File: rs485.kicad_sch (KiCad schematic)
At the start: 4 parts, among them J1 Conn_01x04_Pin, J2 Conn_01x04_Socket, U2 SN74CB3Q3384APW

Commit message: sch of.
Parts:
- removed J2: Conn_01x04_Socket, symbol Connector:Conn_01x04_Socket
- added J2: Conn_01x04_Pin, symbol Connector:Conn_01x04_Pin
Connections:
- net GND: now also J2.1 (Pin_1); no longer J1.4 (Pin_4)
- net at U2.1 (~{1OE}): now also J1.3 (Pin_3)
- net at U2.13 (~{2OE}): now also J1.4 (Pin_4)
- net at U2.2 (1B1): now also J1.1 (Pin_1)
- net at U1.1 (R), U1.4 (D): now also U2.4 (1A2); no longer U2.3 (1A1)
- net at U1.2 (RE~), U1.3 (DE): now also U2.3 (1A1); no longer U2.4 (1A2)
- net at U2.5 (1B2): now also J1.2 (Pin_2)
- net at U1.6 (B): now also J2.3 (Pin_3); no longer J1.2 (Pin_2)
- net at U1.7 (A): now also J2.4 (Pin_4); no longer J1.1 (Pin_1)
- net +5V renamed VCC
- net VCC: now also J2.2 (Pin_2); no longer J1.3 (Pin_3)

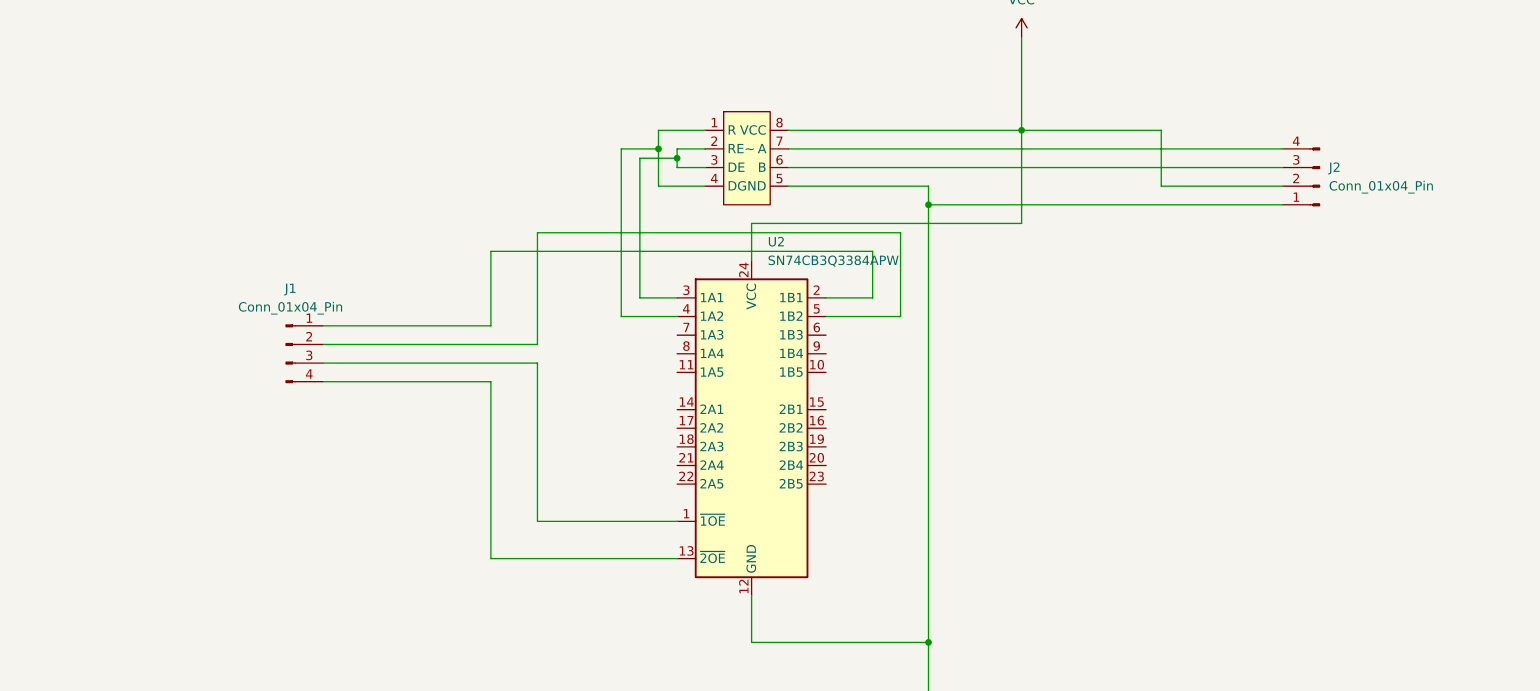
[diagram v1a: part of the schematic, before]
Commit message: sch ok.
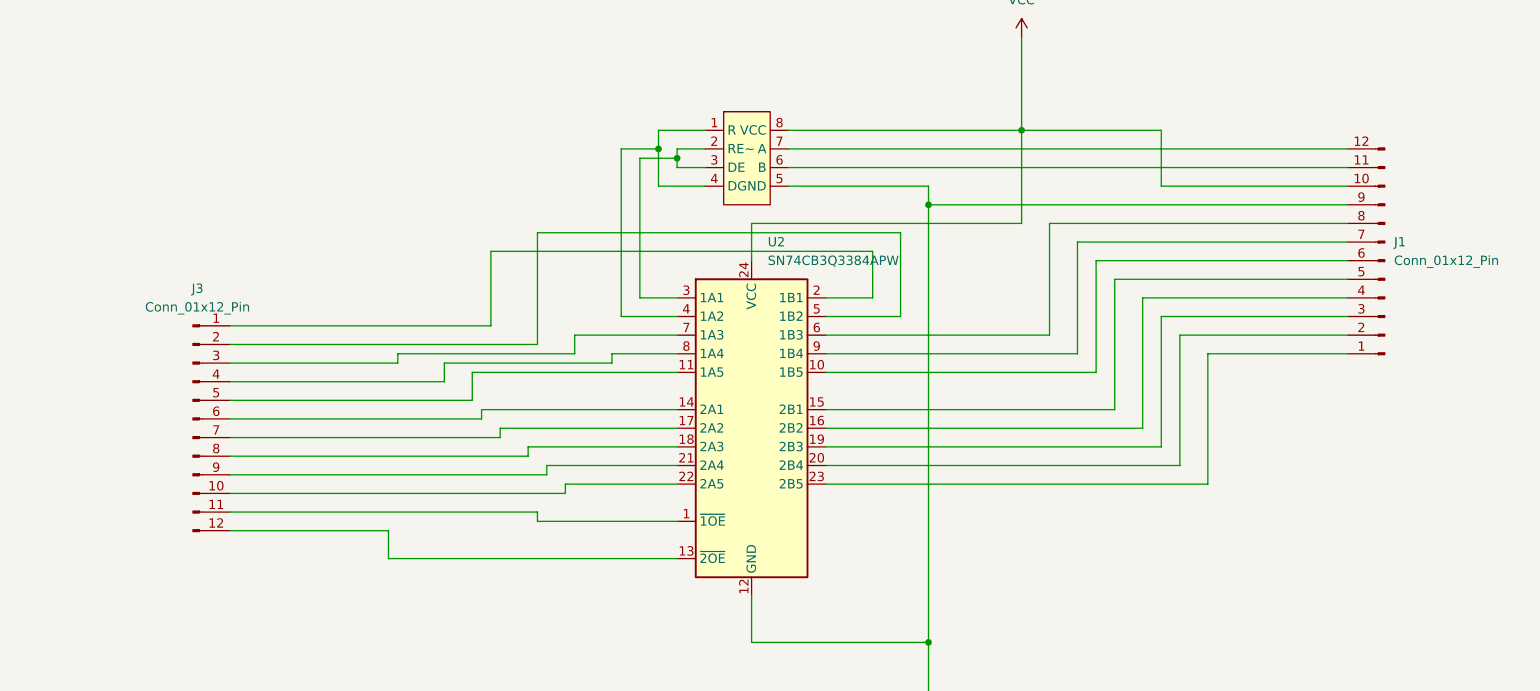
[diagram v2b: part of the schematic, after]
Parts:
- removed J1, J2: Conn_01x04_Pin, symbol Connector:Conn_01x04_Pin
- added J1, J3: Conn_01x12_Pin, symbol Connector:Conn_01x12_Pin
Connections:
- net GND: now also J1.9 (Pin_9)
- net VCC: now also J1.10 (Pin_10)
- net at U1.6 (B): now also J1.11 (Pin_11)
- net at U1.7 (A): now also J1.12 (Pin_12)
- net at U2.2 (1B1): now also J3.1 (Pin_1)
- net at U2.5 (1B2): now also J3.2 (Pin_2)
- net at U2.1 (~{1OE}): now also J3.11 (Pin_11)
- net at U2.13 (~{2OE}): now also J3.12 (Pin_12)
- net at U2.10 (1B5): now also J1.6 (Pin_6)
- net at U2.11 (1A5): now also J3.5 (Pin_5)
- net at U2.14 (2A1): now also J3.6 (Pin_6)
- net at U2.15 (2B1): now also J1.5 (Pin_5)
- net at U2.16 (2B2): now also J1.4 (Pin_4)
- net at U2.17 (2A2): now also J3.7 (Pin_7)
- net at U2.18 (2A3): now also J3.8 (Pin_8)
- net at U2.19 (2B3): now also J1.3 (Pin_3)
- net at U2.20 (2B4): now also J1.2 (Pin_2)
- net at U2.21 (2A4): now also J3.9 (Pin_9)
- net at U2.22 (2A5): now also J3.10 (Pin_10)
- net at U2.23 (2B5): now also J1.1 (Pin_1)
- net at U2.6 (1B3): now also J1.8 (Pin_8)
- net at U2.7 (1A3): now also J3.3 (Pin_3)
- net at U2.8 (1A4): now also J3.4 (Pin_4)
- net at U2.9 (1B4): now also J1.7 (Pin_7)

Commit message: up/.
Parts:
- U1: footprint (none) -> SOIC127P600X175-8N:SOIC127P600X175-8N
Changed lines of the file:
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@@
       (effects (font (size 1.27 1.27)))
     )
-    (property "Footprint" "" (at 114.3 54.61 0)
+    (property "Footprint" "SOIC127P600X175-8N:SOIC127P600X175-8N" (at 114.3 54.61 0)
       (effects (font (size 1.27 1.27)) hide)
     )

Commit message: add pcb file.
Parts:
- J1, J3: footprint (none) -> Connector_PinHeader_2.54mm:PinHeader_1x12_P2.54mm_Vertical
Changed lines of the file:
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@@
       (effects (font (size 1.27 1.27)))
     )
-    (property "Footprint" "" (at 41.91 96.52 0)
+    (property "Footprint" "Connector_PinHeader_2.54mm:PinHeader_1x12_P2.54mm_Vertical" (at 41.91 96.52 0)
       (effects (font (size 1.27 1.27)) hide)
     )
@@
       (effects (font (size 1.27 1.27)) (justify right))
     )
-    (property "Footprint" "" (at 204.47 74.93 0)
+    (property "Footprint" "Connector_PinHeader_2.54mm:PinHeader_1x12_P2.54mm_Vertical" (at 204.47 74.93 0)
       (effects (font (size 1.27 1.27)) hide)
     )
